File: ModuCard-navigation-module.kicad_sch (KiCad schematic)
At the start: 0 parts

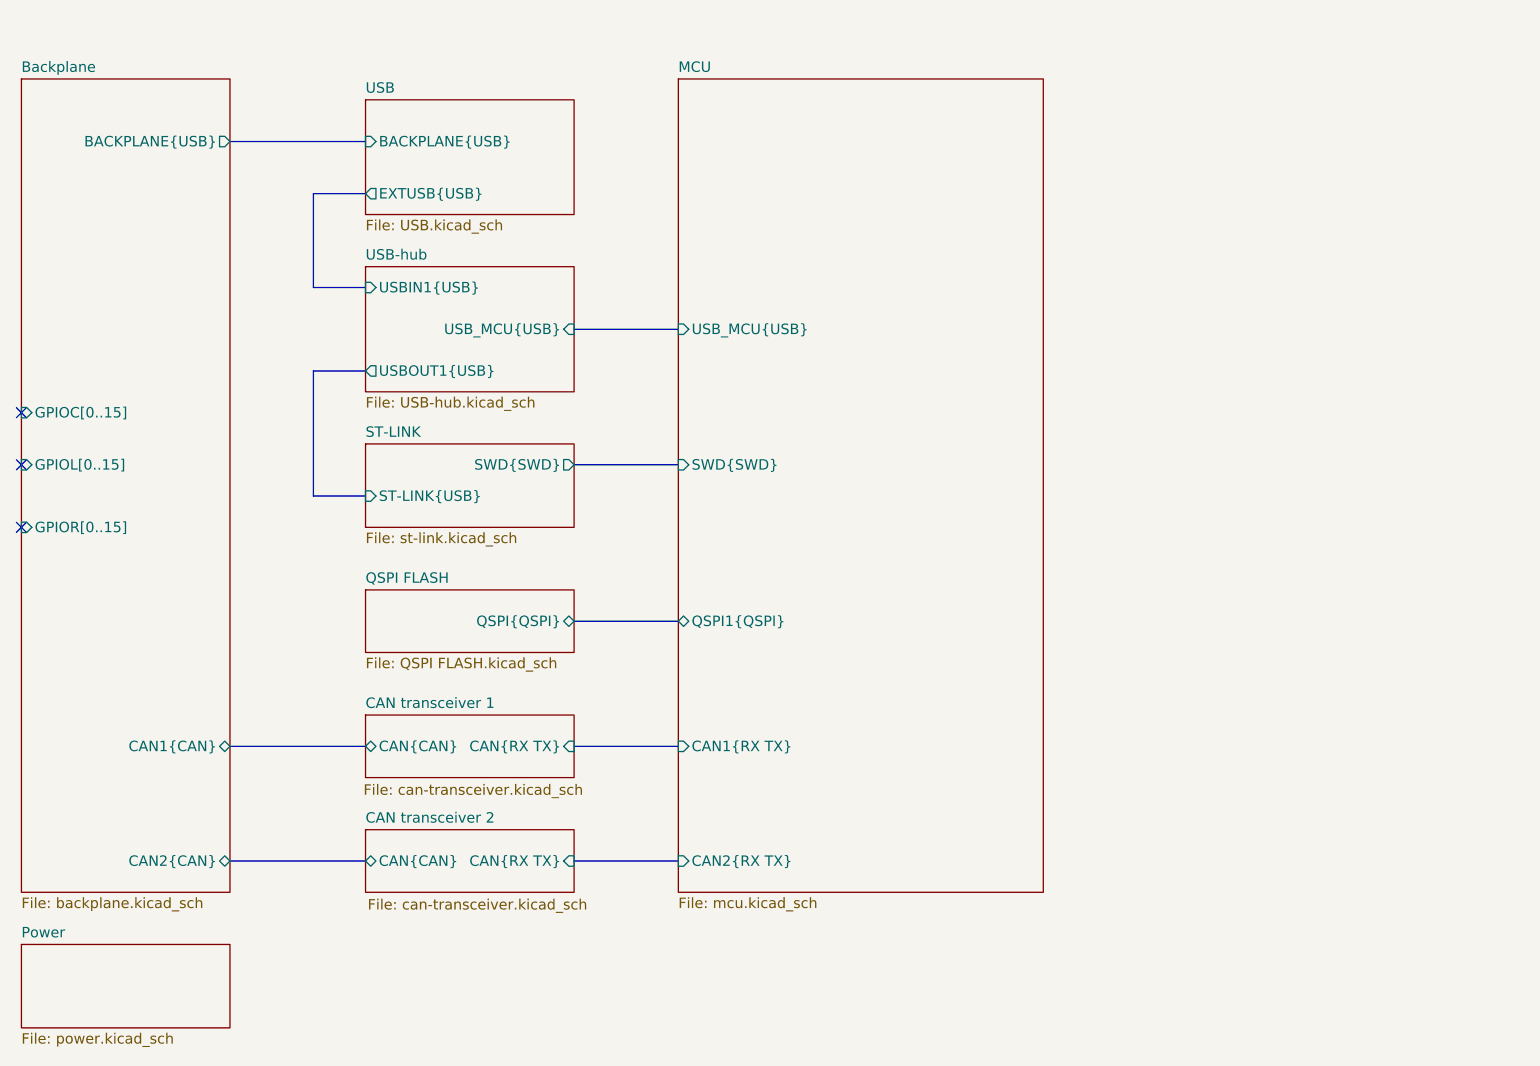
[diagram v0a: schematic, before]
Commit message: [REV2] board finshed, schematics and leyout
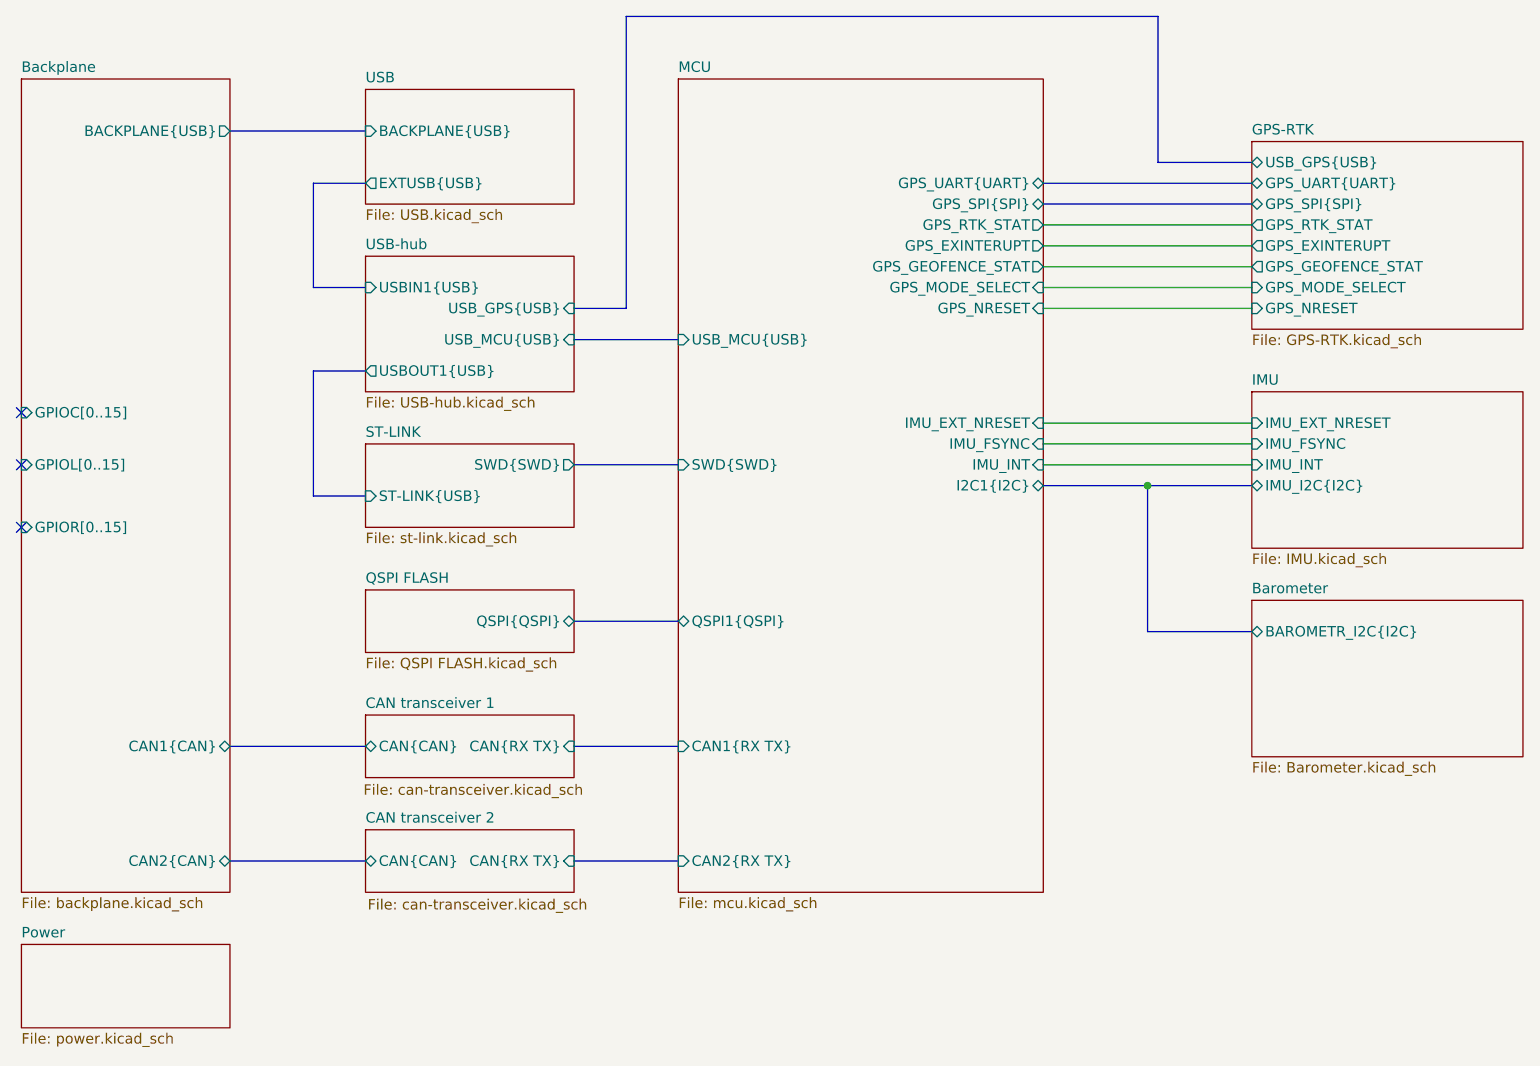
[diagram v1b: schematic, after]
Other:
- added sheet Barometer (Barometer.kicad_sch)
- added sheet GPS-RTK (GPS-RTK.kicad_sch)
- added sheet IMU (IMU.kicad_sch)
- sheet MCU ports: added GPS_EXINTERUPT, GPS_GEOFENCE_STAT, GPS_MODE_SELECT, GPS_NRESET, GPS_RTK_STAT, GPS_SPI{SPI}, GPS_UART{UART}, I2C1{I2C}, IMU_EXT_NRESET, IMU_FSYNC, IMU_INT; removed none
- sheet USB-hub ports: added USB_GPS{USB}; removed none
- title: ModuCard BM STM32H562VGT6 -> ModuCard nav module
